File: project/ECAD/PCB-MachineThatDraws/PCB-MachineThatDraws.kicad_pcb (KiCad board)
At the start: 2 copper layers, 52.5 x 83 mm, 29 parts, among them J1 SD_Card_Device, J10 Conn_02x03_Odd_Even, J11 Conn_02x03_Odd_Even, J2 SDA/SCL/VCC/GND, J3 Switch, J4 Limit_Switch_X, J5 Moteur, J6 Moteur, J7 Barrel_Jack_Switch, J8 Screw_Terminal_01x02, J9 Servo, U1 ESP32-S3-UNO, U2 R-78E5.0-1.0

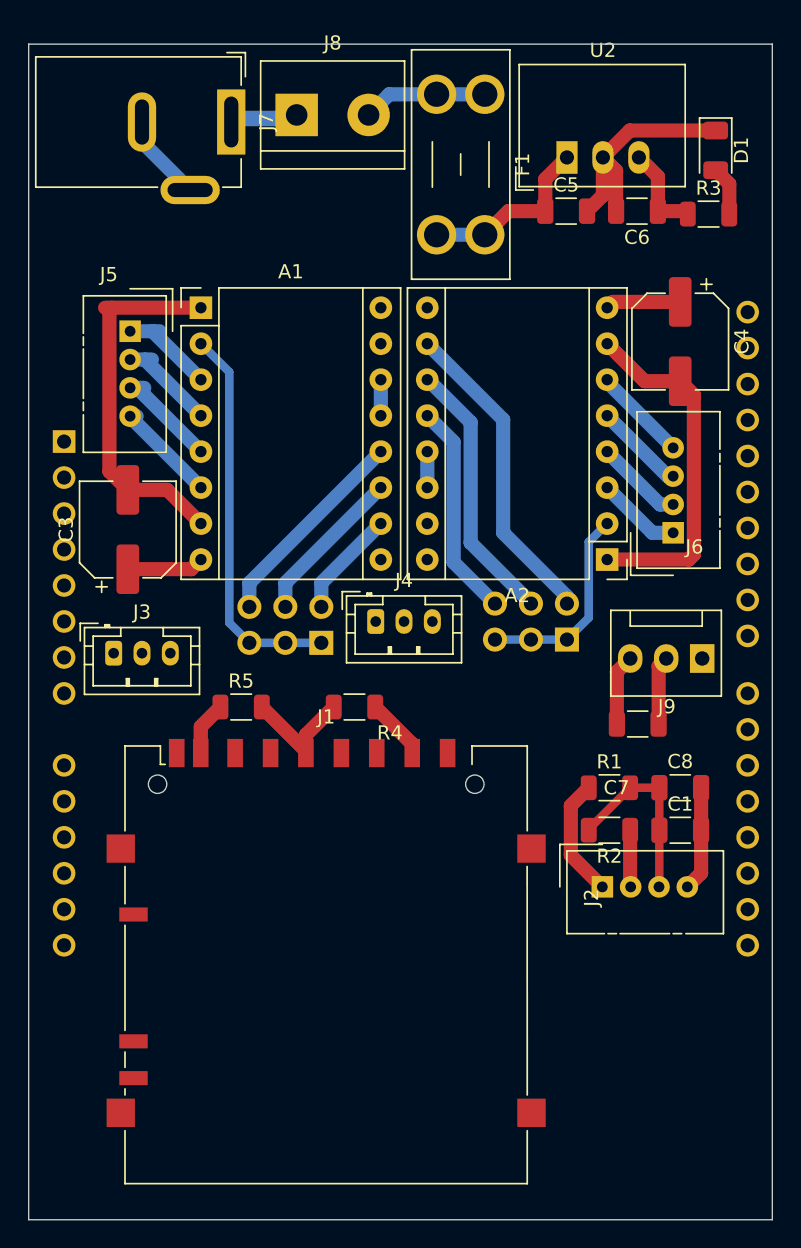
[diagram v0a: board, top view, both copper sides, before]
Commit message: pcb update
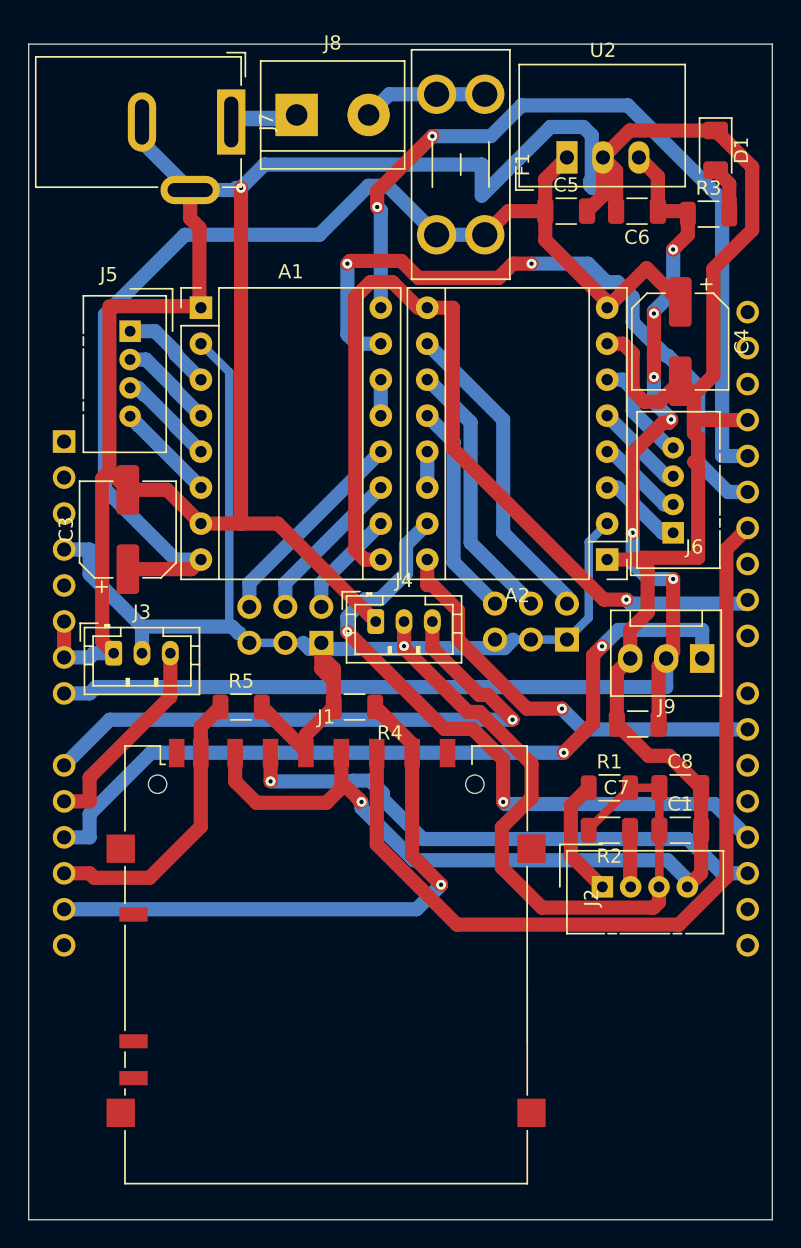
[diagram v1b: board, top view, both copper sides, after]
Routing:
- net GND: track 87.4 -> 279.2 mm, vias 0 -> 2
- net +5V: track 11.4 -> 92.7 mm, vias 0 -> 6
- net +3.3V: track 63.9 -> 144.5 mm, vias 0 -> 1
- net Enable: track 0.00 -> 63.4 mm, vias 0 -> 1
- net +12V: track 23.6 -> 83.8 mm
- net D11: track 0.00 -> 60.1 mm
- net D12: track 0.00 -> 57.8 mm, vias 0 -> 2
- net D07: track 0.00 -> 56.9 mm, vias 0 -> 2
- net D13: track 0.00 -> 47.7 mm, vias 0 -> 2
- net D10: track 0.00 -> 46.6 mm, vias 0 -> 2
- net D9: track 0.00 -> 42.6 mm, vias 0 -> 1
- net D05: track 4.33 -> 43.8 mm, vias 0 -> 1
- net D18: track 0.00 -> 38.7 mm, vias 0 -> 1
- net D14: track 0.00 -> 29.9 mm, vias 0 -> 1
- net D19: track 3.82 -> 21.3 mm
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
